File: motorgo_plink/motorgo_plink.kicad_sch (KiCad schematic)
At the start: 23 parts, among them J1 USB4520-03-0-A_REVA, J4 Conn_02x20_Odd_Even, U1 ESP32-S3-WROOM-1, U2 USBLC6-2P6

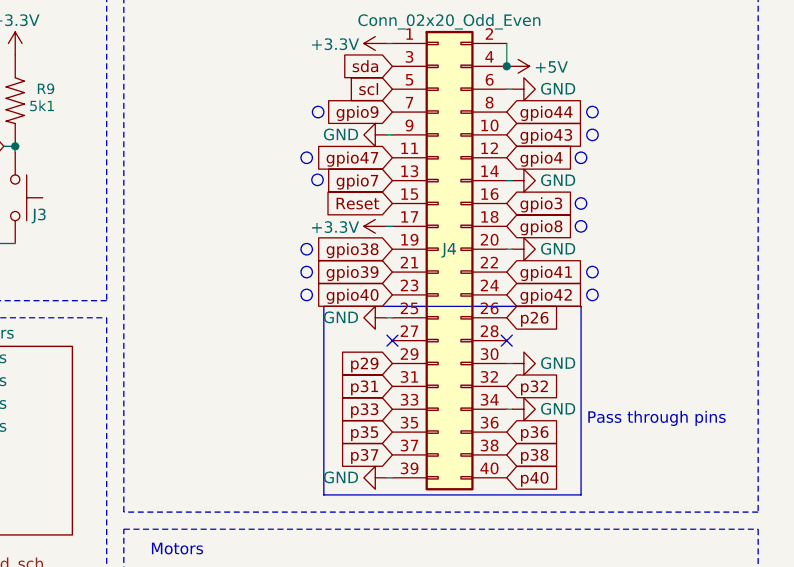
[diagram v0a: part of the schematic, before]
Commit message: WIP update. Layout begin
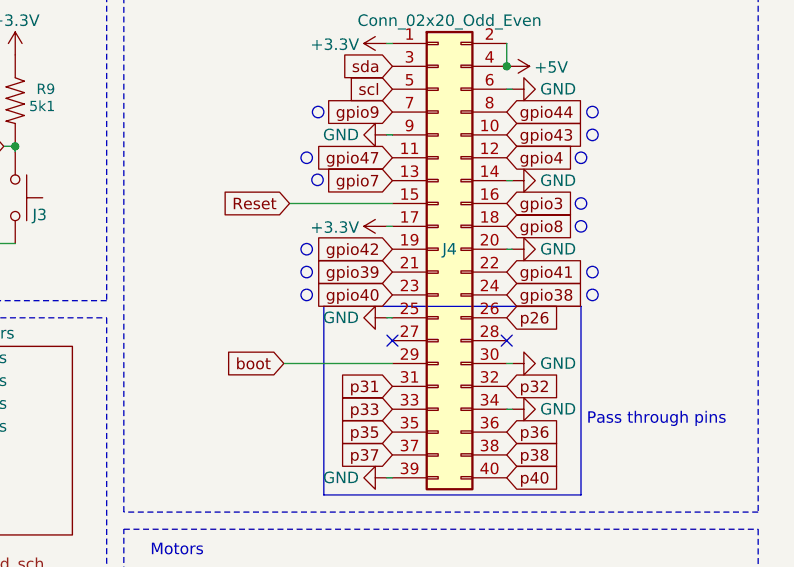
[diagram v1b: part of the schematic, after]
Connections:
- net p29 is gone; now on net boot: J4.29 (Pin_29)
- net gpio38: now also J4.24 (Pin_24); no longer J4.19 (Pin_19)
- net gpio42: now also J4.19 (Pin_19); no longer J4.24 (Pin_24)
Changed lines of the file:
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@@
+    (stroke (width 0) (type default))
+  )
+  (wire (pts (xy 213.995 40.64) (xy 225.425 40.64))
     (stroke (width 0) (type default))
   )
@@
   )
   (polyline (pts (xy 217.805 109.855) (xy 217.17 109.22))
+    (stroke (width 0) (type default))
+  )
+  (wire (pts (xy 213.36 58.42) (xy 225.425 58.42))
     (stroke (width 0) (type default))
   )
@@
     )
   )
-  (global_label "gpio42" (shape input) (at 238.125 50.8 0) (fields_autoplaced)
-    (effects (font (size 1.27 1.27)) (justify left))
-    (property "Intersheetrefs" "${INTERSHEET_REFS}" (at 247.5016 50.8 0)
-      (effects (font (size 1.27 1.27)) (justify left) hide)
+  (global_label "gpio42" (shape input) (at 225.425 45.72 180) (fields_autoplaced)
+    (effects (font (size 1.27 1.27)) (justify right))
+    (property "Intersheetrefs" "${INTERSHEET_REFS}" (at 216.0484 45.72 0)
+      (effects (font (size 1.27 1.27)) (justify right) hide)
     )
   )
@@
     )
   )
+  (global_label "boot" (shape input) (at 213.36 58.42 180) (fields_autoplaced)
+    (effects (font (size 1.27 1.27)) (justify right))
+    (property "Intersheetrefs" "${INTERSHEET_REFS}" (at 206.2815 58.42 0)
+      (effects (font (size 1.27 1.27)) (justify right) hide)
+    )
+  )
   (global_label "m2_PH" (shape input) (at 226.06 112.395 180) (fields_autoplaced)
     (effects (font (size 1.27 1.27) (color 255 255 0 1)) (justify right))
@@
     )
   )
-  (global_label "Reset" (shape input) (at 225.425 40.64 180) (fields_autoplaced)
-    (effects (font (size 1.27 1.27)) (justify right))
-    (property "Intersheetrefs" "${INTERSHEET_REFS}" (at 217.3182 40.64 0)
+  (global_label "Reset" (shape input) (at 213.995 40.64 180) (fields_autoplaced)
+    (effects (font (size 1.27 1.27)) (justify right))
+    (property "Intersheetrefs" "${INTERSHEET_REFS}" (at 205.8882 40.64 0)
       (effects (font (size 1.27 1.27)) (justify right) hide)
     )
@@
     )
   )
-  (global_label "gpio38" (shape input) (at 225.425 45.72 180) (fields_autoplaced)
-    (effects (font (size 1.27 1.27)) (justify right))
-    (property "Intersheetrefs" "${INTERSHEET_REFS}" (at 216.0484 45.72 0)
-      (effects (font (size 1.27 1.27)) (justify right) hide)
+  (global_label "gpio38" (shape input) (at 238.125 50.8 0) (fields_autoplaced)
+    (effects (font (size 1.27 1.27)) (justify left))
+    (property "Intersheetrefs" "${INTERSHEET_REFS}" (at 247.5016 50.8 0)
+      (effects (font (size 1.27 1.27)) (justify left) hide)
     )
   )
@@
     )
   )
-  (global_label "p29" (shape input) (at 225.425 58.42 180) (fields_autoplaced)
-    (effects (font (size 1.27 1.27)) (justify right))
-    (property "Intersheetrefs" "${INTERSHEET_REFS}" (at 218.9512 58.42 0)
-      (effects (font (size 1.27 1.27)) (justify right) hide)
-    )
-  )
